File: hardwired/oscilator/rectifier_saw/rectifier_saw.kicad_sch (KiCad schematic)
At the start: 26 parts, among them Q1 NPN, Q2 PNP, Q4 NPN, Q5 PNP, U1 ${SIM.PARAMS}, U2 ${SIM.PARAMS}, U3 ${SIM.PARAMS}, U4 ${SIM.PARAMS}, U5 ${SIM.PARAMS}

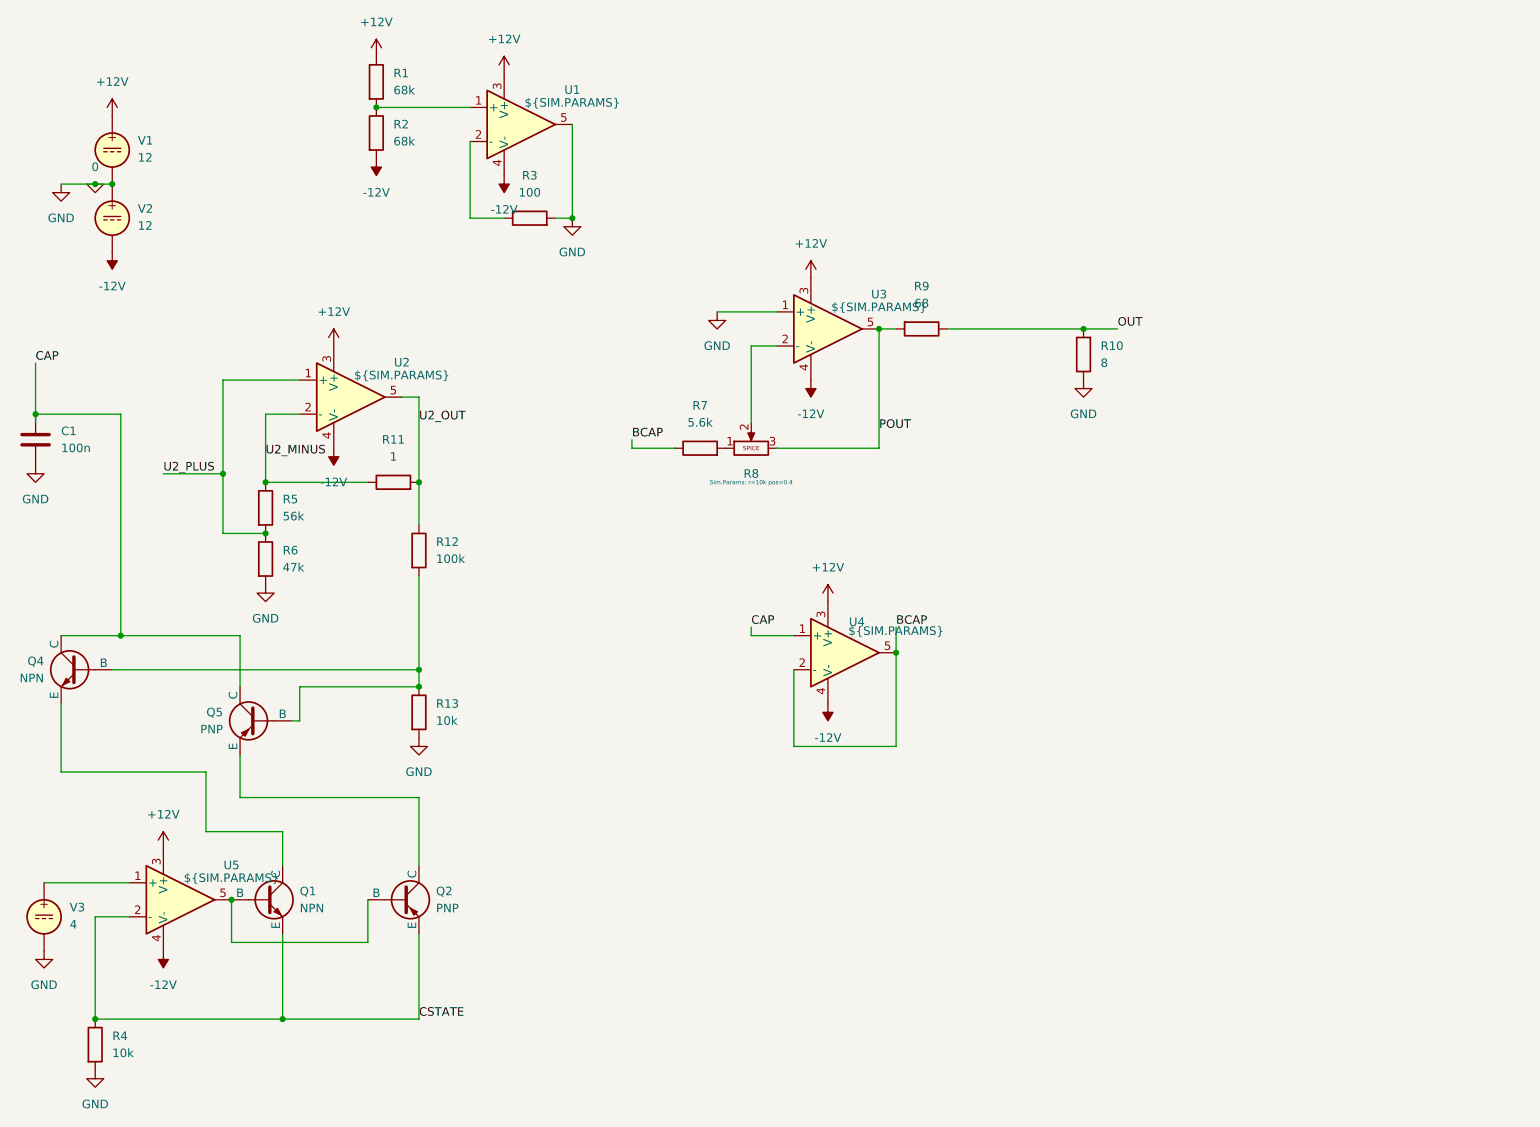
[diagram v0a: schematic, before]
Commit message: Many Kicad drawings
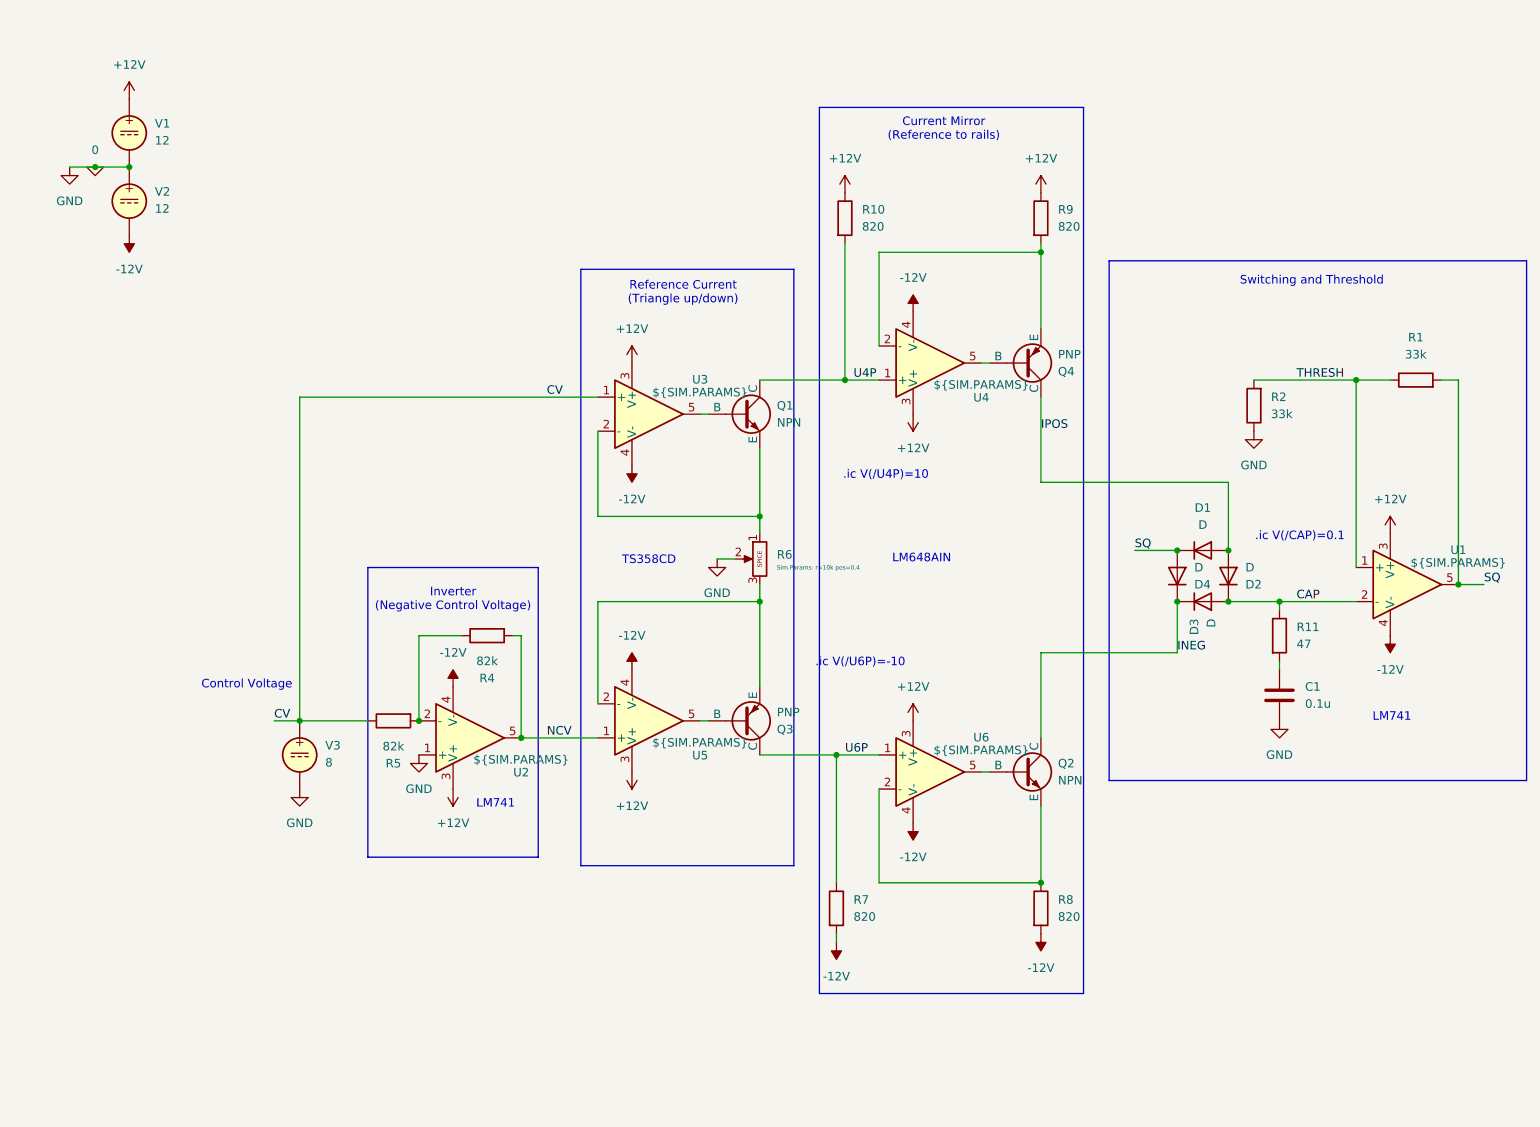
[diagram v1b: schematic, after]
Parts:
- removed Q2, Q5: PNP, symbol Simulation_SPICE:PNP
- removed Q4: NPN, symbol Simulation_SPICE:NPN
- removed R12: 100k, symbol Device:R
- removed R13: 10k, symbol Device:R
- removed R3: 100, symbol Device:R
- removed R6: 47k, symbol Device:R
- removed R8: Potentiometer, symbol Simulation_SPICE:Potentiometer
- added D1, D2, D3, D4: D, symbol Device:D
- added Q2: NPN, symbol Simulation_SPICE:NPN
- added Q3, Q4: PNP, symbol Simulation_SPICE:PNP
- added R6: Potentiometer, symbol Simulation_SPICE:Potentiometer
- added R8: 820, symbol Device:R
- added U6: ${SIM.PARAMS}, symbol Simulation_SPICE:OPAMP
- C1: value 100n -> 0.1u
- R1, R2: value 68k -> 33k
- R10: value 8 -> 820
- R11: value 1 -> 47
- R4: value 10k -> 82k
- R5: value 56k -> 82k
- R7: value 5.6k -> 820
- R9: value 68 -> 820
- V3: value 4 -> 8
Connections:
- net +12V: now also R10.1, R9.1, U6.3 (V+); no longer R1.1
- net -12V: now also R7.2, R8.2, U6.4 (V-); no longer R2.2
- net 0: now also R2.1, U2.1 (+), R6.2; no longer R10.1, R4.2, U1.5, U3.1 (+)
- net CAP: now also R11.1, U1.2 (-), D2.1 (K), D3.2 (A); no longer C1.1, U4.1 (+)
- net CV: now reaches V3.1
- net CV: now also R5.1, U3.1 (+); no longer U5.1 (+)
- net at U3.2 (-): now also Q1.3 (E), R6.1
- net U4P: now reaches Q1.1 (C)
- net U4P: now also R10.2, U4.1 (+)
- net at Q1.2 (B): now also U3.5; no longer U5.5
- removed net BCAP: R7.1, U4.2 (-), U4.5
- removed net CSTATE: Q1.3 (E), R4.1, U5.2 (-)
- removed net OUT: R10.2, R9.1
- net POUT: no longer names the net of R9.2
- net POUT: now also U4.2 (-), Q4.3 (E); no longer U3.5
- removed net U2_MINUS: R11.1, R5.1, U2.2 (-)
- net U2_OUT: no longer names the net of R11.2
- net U2_OUT: now also C1.1; no longer U2.5
- net U2_PLUS: no longer names the net of R5.2
- net U2_PLUS: now also R4.1, U2.2 (-); no longer U2.1 (+)
- new net: Q2.3 (E), R8.1, U6.2 (-)
- new net: Q2.2 (B), U6.5
- new net: Q3.2 (B), U5.5
- new net: Q3.3 (E), R6.3, U5.2 (-)
- new net: Q4.2 (B), U4.5
- new net INEG: D3.1 (K), D4.1 (K), Q2.1 (C)
- new net IPOS: D1.2 (A), D2.2 (A), Q4.1 (C)
- new net NCV: R4.2, U2.5, U5.1 (+)
- new net SQ: D1.1 (K), D4.2 (A), R1.2, U1.5
- new net THRESH: R1.1, R2.2, U1.1 (+)
- new net U6P: Q3.1 (C), R7.1, U6.1 (+)
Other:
- note added: ".ic V(/CAP)=0.1"
- note added: ".ic V(/U4P)=10"
- note added: ".ic V(/U6P)=-10"
- note added: "Control Voltage"
- note added: "Current Mirror (Reference to rails)"
- note added: "Inverter (Negative Control Voltage)"
- note added: "LM648AIN"
- note added: "LM741"
- note added: "Reference Current (Triangle up/down)"
- note added: "Switching and Threshold"
- note added: "TS358CD"
